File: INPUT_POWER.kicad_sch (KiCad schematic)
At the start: 30 parts, among them J1 TYPE-C-31-M12_13, SW3 ON/OFF, U3 IP5306

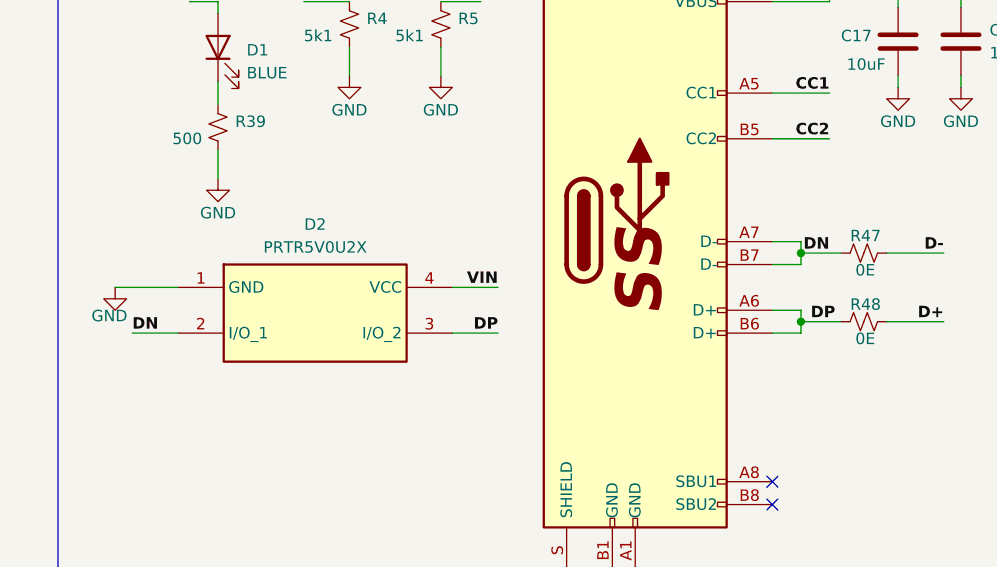
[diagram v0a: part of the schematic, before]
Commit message: Merge changes upstream
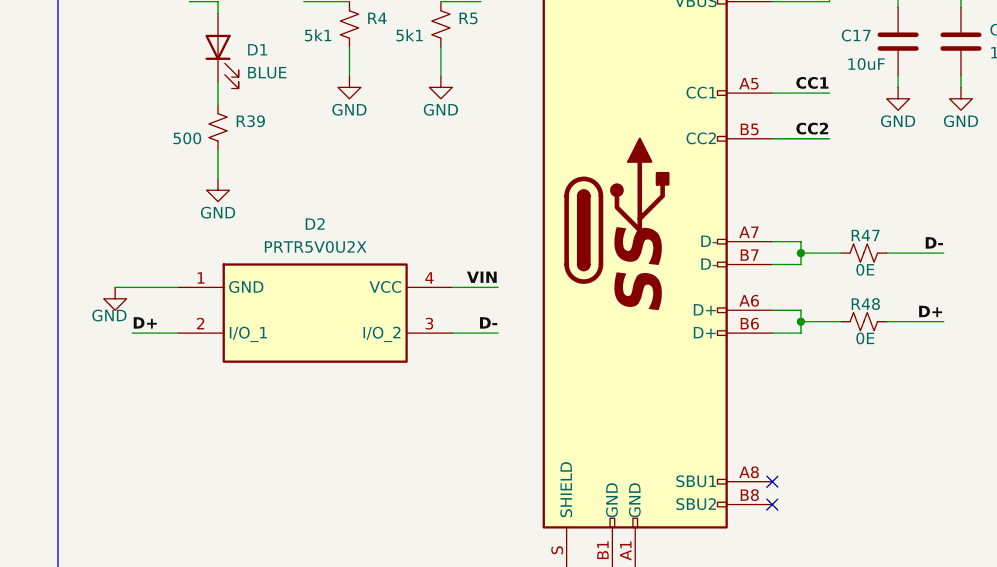
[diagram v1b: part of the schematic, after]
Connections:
- net D+: now also D2.2 (I/O_1)
- net D-: now also D2.3 (I/O_2)
- net DN: no longer names the net of J1.A7 (D-), J1.B7 (D-), R47.1
- net DN: no longer D2.2 (I/O_1)
- net DP: no longer names the net of J1.A6 (D+), J1.B6 (D+), R48.1
- net DP: no longer D2.3 (I/O_2)
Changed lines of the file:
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@@
     (effects (font (size 1.27 1.27) bold (color 0 255 0 1)) (justify left bottom))
   )
-  (label "DN" (at 28.575 95.25 0) (fields_autoplaced)
-    (effects (font (size 1.27 1.27) (thickness 0.254) bold (color 0 0 255 1)) (justify left bottom))
+  (label "D-" (at 69.215 95.25 180) (fields_autoplaced)
+    (effects (font (size 1.27 1.27) (thickness 0.254) bold (color 0 0 255 1)) (justify right bottom))
   )
   (label "V_BAT" (at 38.735 185.42 180) (fields_autoplaced)
@@
     (effects (font (size 1.27 1.27) bold (color 255 0 0 1)) (justify left bottom))
   )
-  (label "DP" (at 106.68 93.98 180) (fields_autoplaced)
-    (effects (font (size 1.27 1.27) (thickness 0.254) bold (color 0 0 255 1)) (justify right bottom))
-  )
   (label "VIN" (at 69.215 90.17 180) (fields_autoplaced)
     (effects (font (size 1.27 1.27) (thickness 0.254) bold (color 255 0 0 1)) (justify right bottom))
@@
     (effects (font (size 1.27 1.27) (thickness 0.254) bold (color 255 0 0 1)) (justify left bottom))
   )
-  (label "DP" (at 69.215 95.25 180) (fields_autoplaced)
-    (effects (font (size 1.27 1.27) (thickness 0.254) bold (color 0 0 255 1)) (justify right bottom))
+  (label "D+" (at 28.575 95.25 0) (fields_autoplaced)
+    (effects (font (size 1.27 1.27) (thickness 0.254) bold (color 0 0 255 1)) (justify left bottom))
   )
   (label "VOUT" (at 274.955 73.025 180) (fields_autoplaced)
@@
     (effects (font (size 1.27 1.27) bold (color 0 255 0 1)) (justify left bottom))
   )
-  (label "DN" (at 106.045 86.36 180) (fields_autoplaced)
-    (effects (font (size 1.27 1.27) (thickness 0.254) bold (color 0 0 255 1)) (justify right bottom))
-  )
   (label "CC2" (at 67.31 58.42 180) (fields_autoplaced)
